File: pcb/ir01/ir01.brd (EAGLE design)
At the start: 65 x 30.5 mm, 9 parts

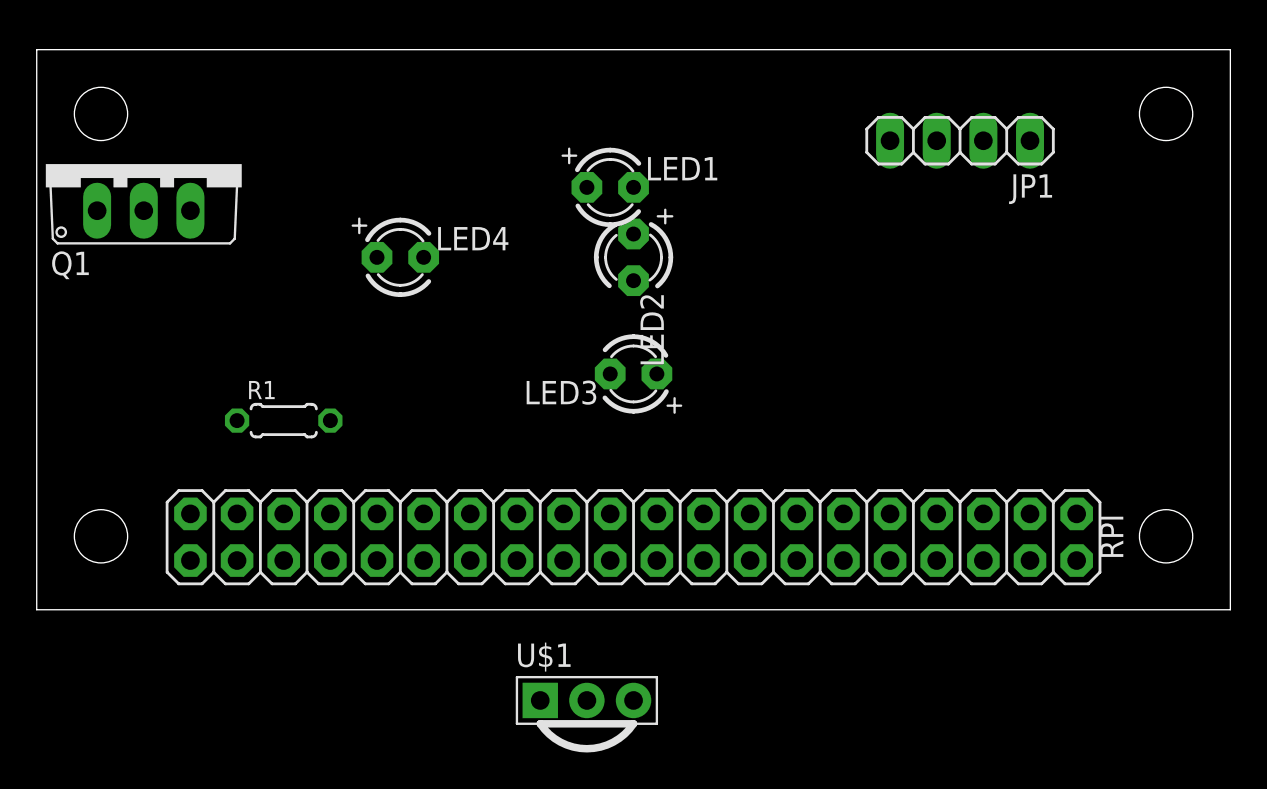
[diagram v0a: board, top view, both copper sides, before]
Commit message: pcb
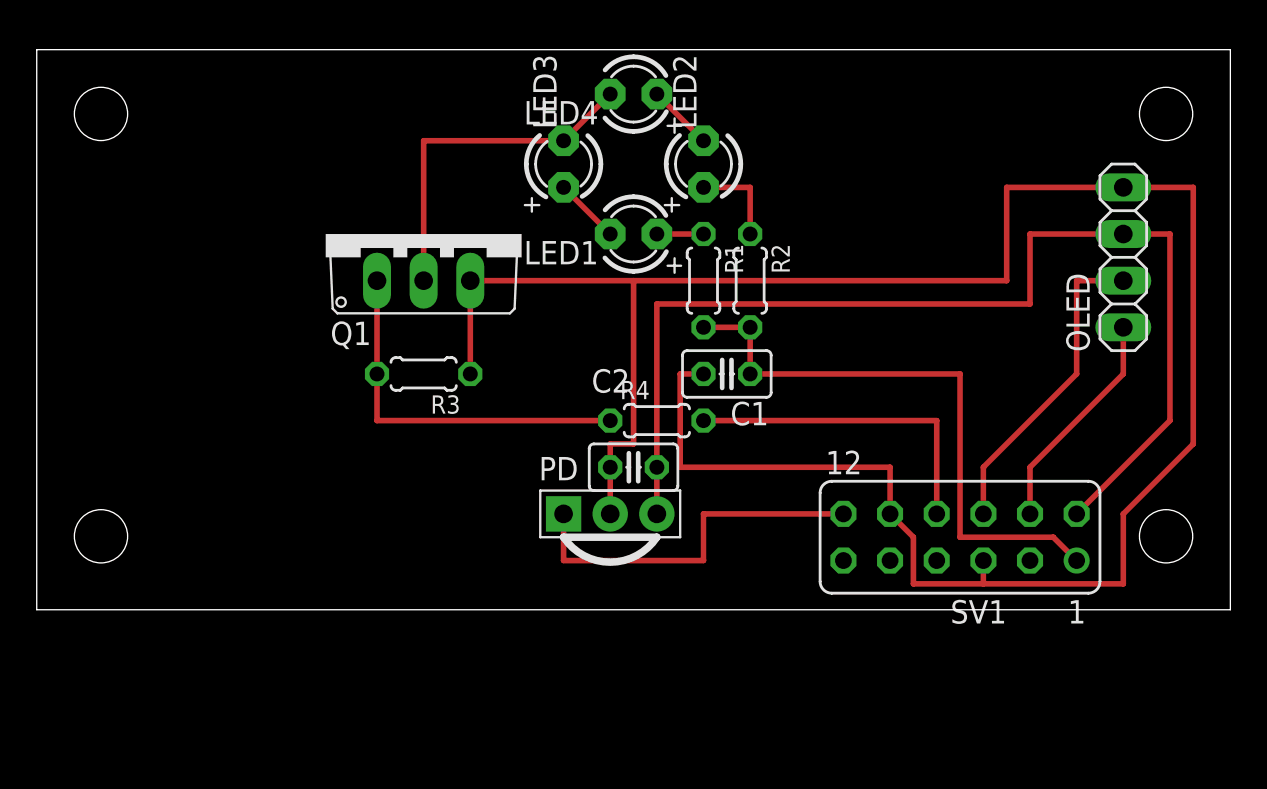
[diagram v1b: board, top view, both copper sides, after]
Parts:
- removed JP1: (no value), pinhead:1X04
- removed RPI: (no value), adafruit:2X20-BIG
- removed U$1: PNA460XM, adafruit:PNA460XM
- added C1: 47uF, rcl:C025-025X050
- added C2: 0.1μF, rcl:C025-025X050
- added OLED: (no value), pinhead:1X04
- added PD: OSRB38C9AA, adafruit:PNA460XM
- added R2: 10Ω, rcl:0204/5
- added R3: 10kΩ, rcl:0204/5
- added R4: 330Ω, rcl:0204/5
- added SV1: (no value), con-lsta:FE06-2
- R1: value (none) -> 10Ω
- moved R1 24.1 mm to (38.1, 20.3), turned to 270 degrees
- moved Q1 15.7 mm to (22.9, 22.9)
- moved LED4 15.5 mm to (34.3, 30.5), turned to 180 degrees
- moved LED3 12.0 mm to (30.5, 26.7), turned to 90 degrees
- moved LED2 6.35 mm to (38.1, 26.7), turned to 90 degrees
- moved LED1 2.84 mm to (34.3, 22.9), turned to 180 degrees
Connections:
- removed net N$6: RPI.2, RPI.4
- removed net VCC: U$1.3
- new net 3.3V: C2.1, OLED.3, PD.3, SV1.2
- new net 5V: C1.1, R1.2, R2.2, SV1.1
- new net N$4: LED1.A, R1.1
- new net N$5: LED2.A, R2.1
- new net N$7: LED1.K, LED3.A
- new net N$8: LED2.K, LED4.A
- new net N$9: LED3.K, LED4.K, Q1.2
- new net SDA: OLED.1, SV1.4
- new net SDC: OLED.2, SV1.6
- net GND: now also C1.2, C2.2, OLED.4, PD.2, Q1.3, R3.1, SV1.10, SV1.5; no longer JP1.4, RPI.14, RPI.20, RPI.25, RPI.30, RPI.34, RPI.39, RPI.6, RPI.9, U$1.2
- net N$1: now also Q1.1, R3.2, R4.1; no longer JP1.1, RPI.1, RPI.17
- net N$2: now also PD.1, SV1.12; no longer JP1.2, RPI.3
- net N$3: now also R4.2, SV1.8; no longer JP1.3, RPI.5
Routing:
- net GND: track 0.00 -> 124.0 mm
- net 3.3V: track 0.00 -> 60.5 mm
- net 5V: track 0.00 -> 32.3 mm
- net N$1: track 0.00 -> 20.3 mm
- net N$2: track 0.00 -> 20.3 mm
- net N$9: track 0.00 -> 18.8 mm
- net N$3: track 0.00 -> 17.8 mm
- net SDC: track 0.00 -> 17.3 mm
- net SDA: track 0.00 -> 12.3 mm
- net N$5: track 0.00 -> 5.08 mm
- net N$7: track 0.00 -> 3.59 mm
- net N$8: track 0.00 -> 3.59 mm
- net N$4: track 0.00 -> 2.54 mm
